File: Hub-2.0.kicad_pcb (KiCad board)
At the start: 2 copper layers, 120 x 78 mm, 9 parts, among them CN1 6437288-3, CN4 DT15-12PA, CN5 DT15-12PA, CN6 DT15-12PA, J3-PCB1 5569-06A2, U1 YQ506-S-112 DM

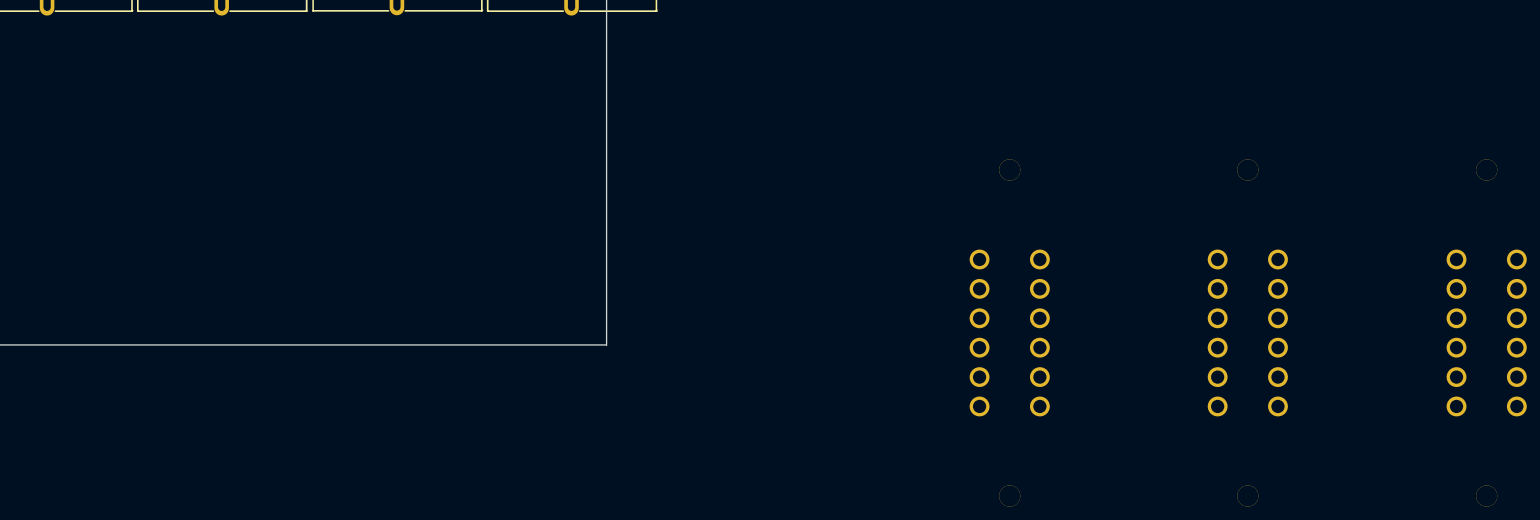
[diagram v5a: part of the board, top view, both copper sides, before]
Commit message: Autosave
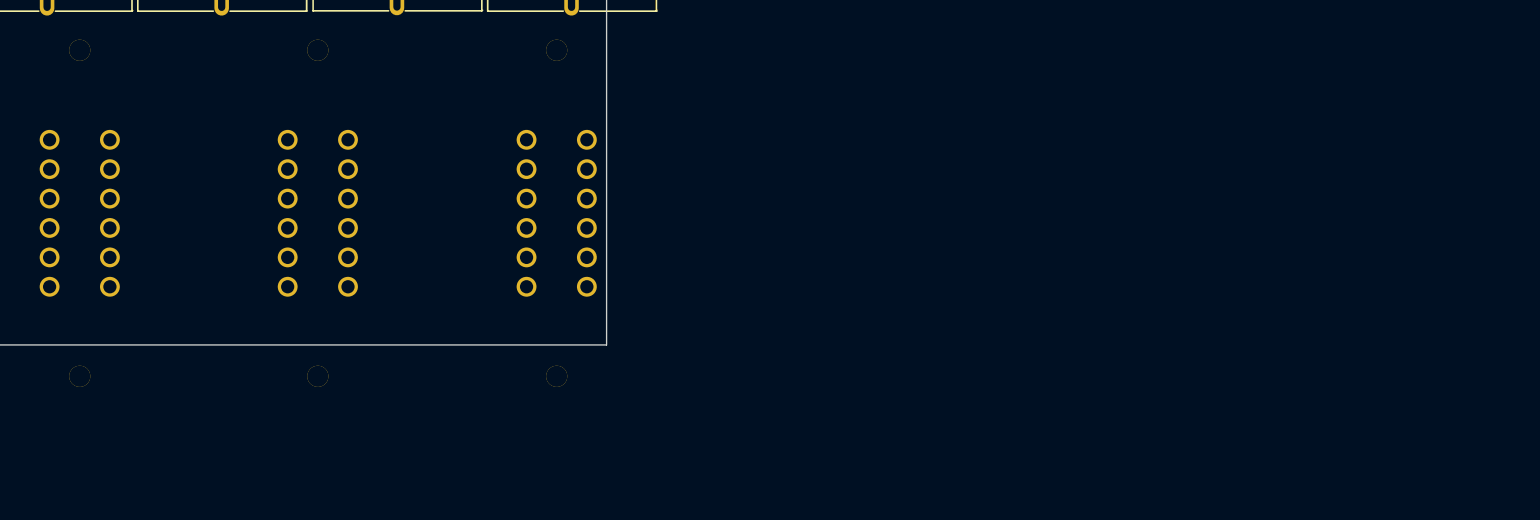
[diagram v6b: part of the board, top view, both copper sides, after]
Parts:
- moved CN4 141.8 mm to (161.6, 86.9)
- moved CN5 141.8 mm to (125.4, 86.9)
- moved CN6 141.8 mm to (89.4, 86.9)
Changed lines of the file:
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@@
 	(footprint "EasyEDA:CONN-TH_DT15-12PA"
 		(layer "B.Cu")
-		(at 266.06 104.99 180)
+		(at 125.44 86.89 180)
 		(property "Reference" "CN5"
 			(at 0 15.109999 0)
@@
 	(footprint "EasyEDA:CONN-TH_DT15-12PA"
 		(layer "B.Cu")
-		(at 302.18 104.99 180)
+		(at 161.56 86.89 180)
 		(property "Reference" "CN4"
 			(at 0 15.109999 0)
@@
 	(footprint "EasyEDA:CONN-TH_DT15-12PA"
 		(layer "B.Cu")
-		(at 230.06 104.99 180)
+		(at 89.44 86.89 180)
 		(property "Reference" "CN6"
 			(at 0 15.109999 0)
